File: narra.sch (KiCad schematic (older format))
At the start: 8 parts

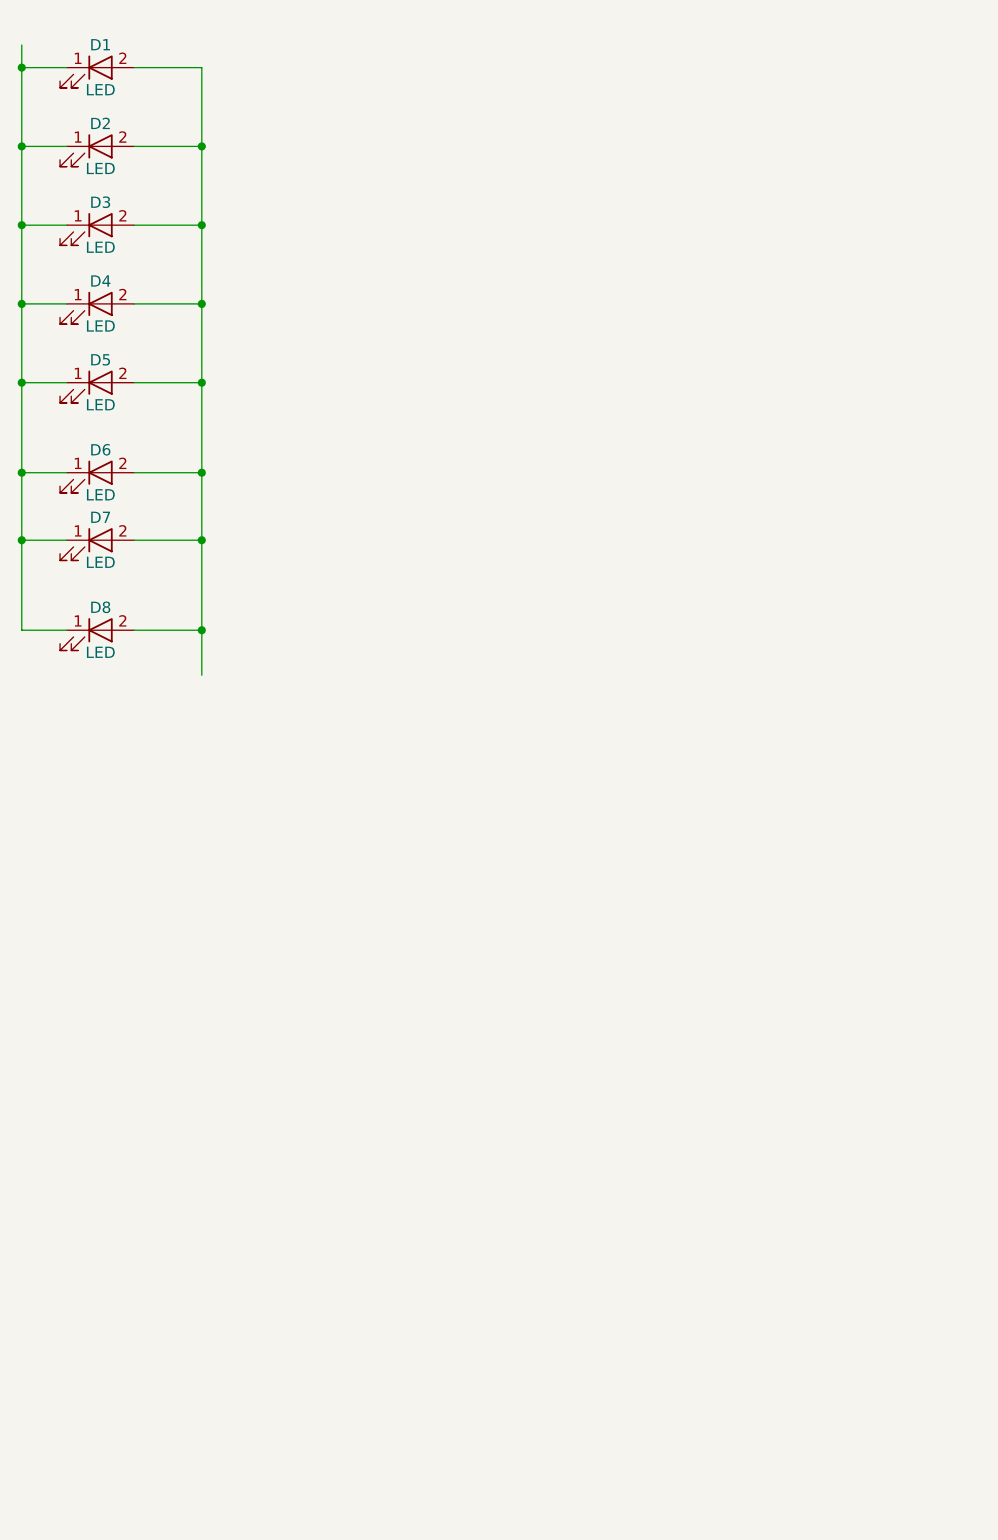
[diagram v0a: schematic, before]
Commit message: Changed LED footprint to suit the schematic
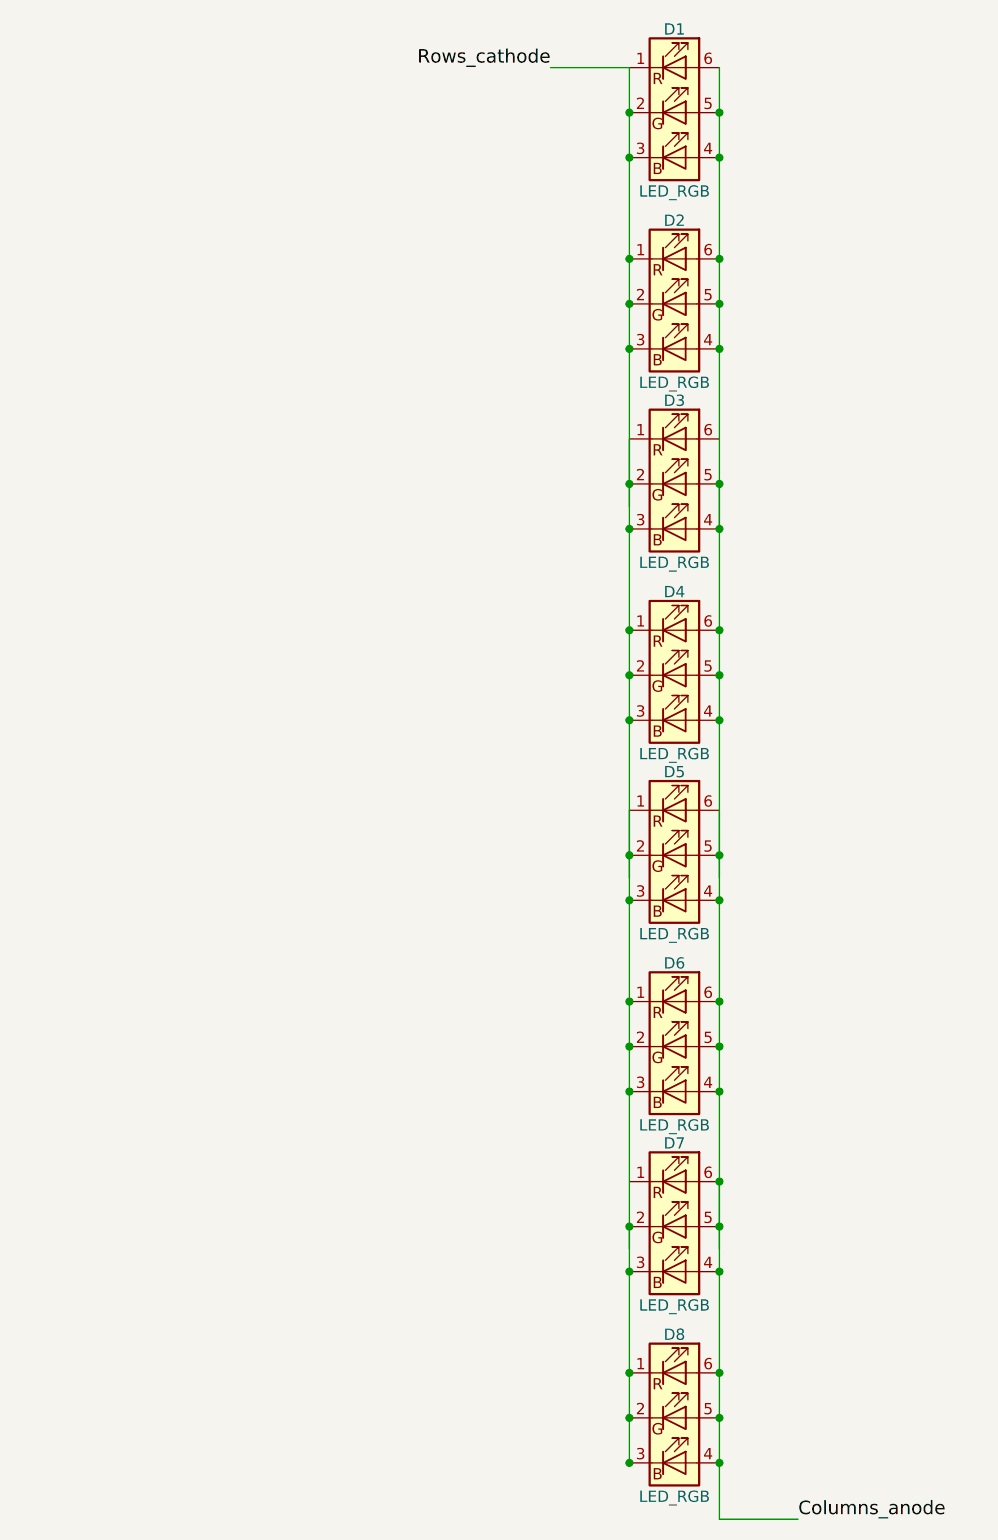
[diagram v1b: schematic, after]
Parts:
- removed D1, D2, D3, D4, D5, D6, D7, D8: LED, LEDs:LED_PLCC_2835, symbol LED
- added D1, D2, D3, D4, D5, D6, D7, D8: LED_RGB, LEDs:LED_WS2812-PLCC6, symbol LED_RGB
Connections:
- net labels added: Columns_anode, Rows_cathode
- wire segments 18 -> 10
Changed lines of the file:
@@
 $EndDescr
 $Comp
-L LED D1
-U 1 1 58D2CCCA
-P 1350 800
-F 0 "D1" H 1350 900 50  0000 C CNN
-F 1 "LED" H 1350 700 50  0000 C CNN
-F 2 "LEDs:LED_PLCC_2835" H 1350 800 50  0001 C CNN
-F 3 "" H 1350 800 50  0000 C CNN
-	1    1350 800
+L LED_RGB D1
+U 1 1 58DE0E2B
+P 3900 1000
+F 0 "D1" H 3900 1370 50  0000 C CNN
+F 1 "LED_RGB" H 3900 650 50  0000 C CNN
+F 2 "LEDs:LED_WS2812-PLCC6" H 3900 950 50  0001 C CNN
+F 3 "" H 3900 950 50  0001 C CNN
+	1    3900 1000
 	1    0    0    -1
 $EndComp
 $Comp
-L LED D2
-U 1 1 58D2CE12
-P 1350 1150
-F 0 "D2" H 1350 1250 50  0000 C CNN
-F 1 "LED" H 1350 1050 50  0000 C CNN
-F 2 "LEDs:LED_PLCC_2835" H 1350 1150 50  0001 C CNN
-F 3 "" H 1350 1150 50  0000 C CNN
-	1    1350 1150
+L LED_RGB D2
+U 1 1 58DE0E90
+P 3900 1850
+F 0 "D2" H 3900 2220 50  0000 C CNN
+F 1 "LED_RGB" H 3900 1500 50  0000 C CNN
+F 2 "LEDs:LED_WS2812-PLCC6" H 3900 1800 50  0001 C CNN
+F 3 "" H 3900 1800 50  0001 C CNN
+	1    3900 1850
 	1    0    0    -1
 $EndComp
 $Comp
-L LED D3
-U 1 1 58D2CE37
-P 1350 1500
-F 0 "D3" H 1350 1600 50  0000 C CNN
-F 1 "LED" H 1350 1400 50  0000 C CNN
-F 2 "LEDs:LED_PLCC_2835" H 1350 1500 50  0001 C CNN
-F 3 "" H 1350 1500 50  0000 C CNN
-	1    1350 1500
+L LED_RGB D3
+U 1 1 58DE125F
+P 3900 2650
+F 0 "D3" H 3900 3020 50  0000 C CNN
+F 1 "LED_RGB" H 3900 2300 50  0000 C CNN
+F 2 "LEDs:LED_WS2812-PLCC6" H 3900 2600 50  0001 C CNN
+F 3 "" H 3900 2600 50  0001 C CNN
+	1    3900 2650
 	1    0    0    -1
 $EndComp
 $Comp
-L LED D4
-U 1 1 58D2CE4E
-P 1350 1850
-F 0 "D4" H 1350 1950 50  0000 C CNN
-F 1 "LED" H 1350 1750 50  0000 C CNN
-F 2 "LEDs:LED_PLCC_2835" H 1350 1850 50  0001 C CNN
-F 3 "" H 1350 1850 50  0000 C CNN
-	1    1350 1850
+L LED_RGB D4
+U 1 1 58DE1265
+P 3900 3500
+F 0 "D4" H 3900 3870 50  0000 C CNN
+F 1 "LED_RGB" H 3900 3150 50  0000 C CNN
+F 2 "LEDs:LED_WS2812-PLCC6" H 3900 3450 50  0001 C CNN
+F 3 "" H 3900 3450 50  0001 C CNN
+	1    3900 3500
 	1    0    0    -1
 $EndComp
 $Comp
-L LED D5
-U 1 1 58D2CE67
-P 1350 2200
-F 0 "D5" H 1350 2300 50  0000 C CNN
-F 1 "LED" H 1350 2100 50  0000 C CNN
-F 2 "LEDs:LED_PLCC_2835" H 1350 2200 50  0001 C CNN
-F 3 "" H 1350 2200 50  0000 C CNN
-	1    1350 2200
+L LED_RGB D5
+U 1 1 58DE1E6F
+P 3900 4300
+F 0 "D5" H 3900 4670 50  0000 C CNN
+F 1 "LED_RGB" H 3900 3950 50  0000 C CNN
+F 2 "LEDs:LED_WS2812-PLCC6" H 3900 4250 50  0001 C CNN
+F 3 "" H 3900 4250 50  0001 C CNN
+	1    3900 4300
 	1    0    0    -1
 $EndComp
 $Comp
-L LED D6
-U 1 1 58D2CE82
-P 1350 2600
-F 0 "D6" H 1350 2700 50  0000 C CNN
-F 1 "LED" H 1350 2500 50  0000 C CNN
-F 2 "LEDs:LED_PLCC_2835" H 1350 2600 50  0001 C CNN
-F 3 "" H 1350 2600 50  0000 C CNN
-	1    1350 2600
+L LED_RGB D6
+U 1 1 58DE1E75
+P 3900 5150
+F 0 "D6" H 3900 5520 50  0000 C CNN
+F 1 "LED_RGB" H 3900 4800 50  0000 C CNN
+F 2 "LEDs:LED_WS2812-PLCC6" H 3900 5100 50  0001 C CNN
+F 3 "" H 3900 5100 50  0001 C CNN
+	1    3900 5150
 	1    0    0    -1
 $EndComp
 $Comp
-L LED D7
-U 1 1 58D2CE9F
-P 1350 2900
-F 0 "D7" H 1350 3000 50  0000 C CNN
-F 1 "LED" H 1350 2800 50  0000 C CNN
-F 2 "LEDs:LED_PLCC_2835" H 1350 2900 50  0001 C CNN
-F 3 "" H 1350 2900 50  0000 C CNN
-	1    1350 2900
+L LED_RGB D7
+U 1 1 58DE1E87
+P 3900 5950
+F 0 "D7" H 3900 6320 50  0000 C CNN
+F 1 "LED_RGB" H 3900 5600 50  0000 C CNN
+F 2 "LEDs:LED_WS2812-PLCC6" H 3900 5900 50  0001 C CNN
+F 3 "" H 3900 5900 50  0001 C CNN
+	1    3900 5950
 	1    0    0    -1
 $EndComp
 $Comp
-L LED D8
-U 1 1 58D2CEBE
-P 1350 3300
-F 0 "D8" H 1350 3400 50  0000 C CNN
-F 1 "LED" H 1350 3200 50  0000 C CNN
-F 2 "LEDs:LED_PLCC_2835" H 1350 3300 50  0001 C CNN
-F 3 "" H 1350 3300 50  0000 C CNN
-	1    1350 3300
+L LED_RGB D8
+U 1 1 58DE1E8D
+P 3900 6800
+F 0 "D8" H 3900 7170 50  0000 C CNN
+F 1 "LED_RGB" H 3900 6450 50  0000 C CNN
+F 2 "LEDs:LED_WS2812-PLCC6" H 3900 6750 50  0001 C CNN
+F 3 "" H 3900 6750 50  0001 C CNN
+	1    3900 6800
 	1    0    0    -1
 $EndComp
 Wire Wire Line
-	1000 700  1000 3300
+	3700 800  3700 2750
+Connection ~ 3700 1000
+Connection ~ 3700 1200
+Connection ~ 3700 1650
+Connection ~ 3700 1850
+Connection ~ 3700 2050
 Wire Wire Line
-	1800 3500 1800 800
+	4100 800  4100 2850
+Connection ~ 4100 1000
+Connection ~ 4100 1650
+Connection ~ 4100 1850
+Connection ~ 4100 2050
 Wire Wire Line
-	1200 800  1000 800
-Connection ~ 1000 800
+	3700 2450 3700 4400
+Connection ~ 3700 2650
+Connection ~ 3700 2850
+Connection ~ 3700 3300
+Connection ~ 3700 3500
+Connection ~ 3700 3700
+Connection ~ 4100 2650
 Wire Wire Line
-	1200 1150 1000 1150
-Connection ~ 1000 1150
+	4100 2650 4100 4400
+Connection ~ 4100 3300
+Connection ~ 4100 3500
+Connection ~ 4100 3700
 Wire Wire Line
-	1200 1500 1000 1500
-Connection ~ 1000 1500
+	3700 4100 3700 6050
+Connection ~ 3700 4300
+Connection ~ 3700 4500
+Connection ~ 3700 4950
+Connection ~ 3700 5150
+Connection ~ 3700 5350
+Connection ~ 4100 4300
+Connection ~ 4100 4950
+Connection ~ 4100 5150
+Connection ~ 4100 5350
+Connection ~ 3700 5950
+Connection ~ 3700 6150
+Connection ~ 3700 6600
+Connection ~ 3700 6800
+Connection ~ 3700 7000
+Connection ~ 4100 5950
+Connection ~ 4100 6600
+Connection ~ 4100 6800
+Connection ~ 4100 7000
+Connection ~ 4100 1200
+Connection ~ 4100 2850
+Connection ~ 4100 4500
+Connection ~ 4100 6150
 Wire Wire Line
-	1200 1850 1000 1850
-Connection ~ 1000 1850
+	4100 4100 4100 6050
 Wire Wire Line
-	1200 2200 1000 2200
-Connection ~ 1000 2200
+	4100 5750 4100 7250
 Wire Wire Line
-	1200 2600 1000 2600
-Connection ~ 1000 2600
+	3700 7000 3700 5950
+Connection ~ 4100 5750
 Wire Wire Line
-	1200 2900 1000 2900
-Connection ~ 1000 2900
+	3700 800  3350 800
 Wire Wire Line
-	1000 3300 1200 3300
-Wire Wire Line
-	1800 800  1500 800
-Wire Wire Line
-	1500 1150 1800 1150
-Connection ~ 1800 1150
-Wire Wire Line
-	1500 1500 1800 1500
-Connection ~ 1800 1500
-Wire Wire Line
-	1500 1850 1800 1850
-Connection ~ 1800 1850
-Wire Wire Line
-	1500 2200 1800 2200
-Connection ~ 1800 2200
-Wire Wire Line
-	1500 2600 1800 2600
-Connection ~ 1800 2600
-Wire Wire Line
-	1500 2900 1800 2900
-Connection ~ 1800 2900
-Wire Wire Line
-	1500 3300 1800 3300
-Connection ~ 1800 3300
+	4100 7250 4450 7250
+Text Label 3350 800  2    60   ~ 0
+Rows_cathode
+Text Label 4450 7250 0    60   ~ 0
+Columns_anode
 $EndSCHEMATC
